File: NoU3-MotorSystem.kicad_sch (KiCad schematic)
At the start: 26 parts, among them J15 Barrel_Jack, J16 VIN, J18 GND, Q2 AONR21357, U15 SY8113BADC, U16 SY8113BADC, U8 5.8 ZSPT

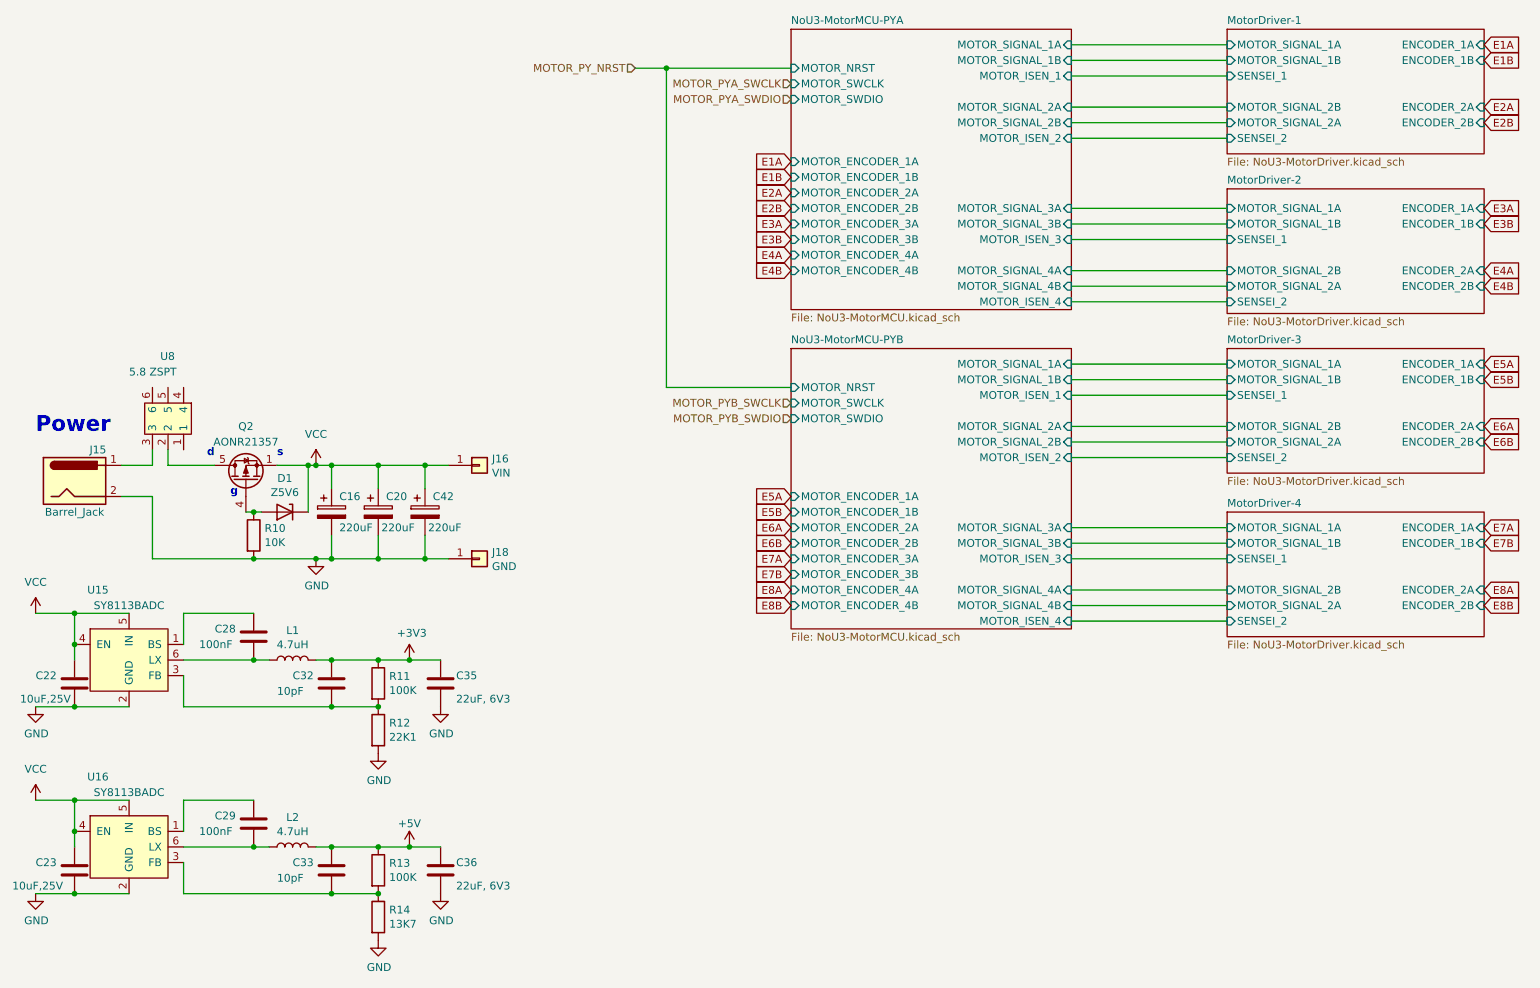
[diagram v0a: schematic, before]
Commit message: motor driver footprints
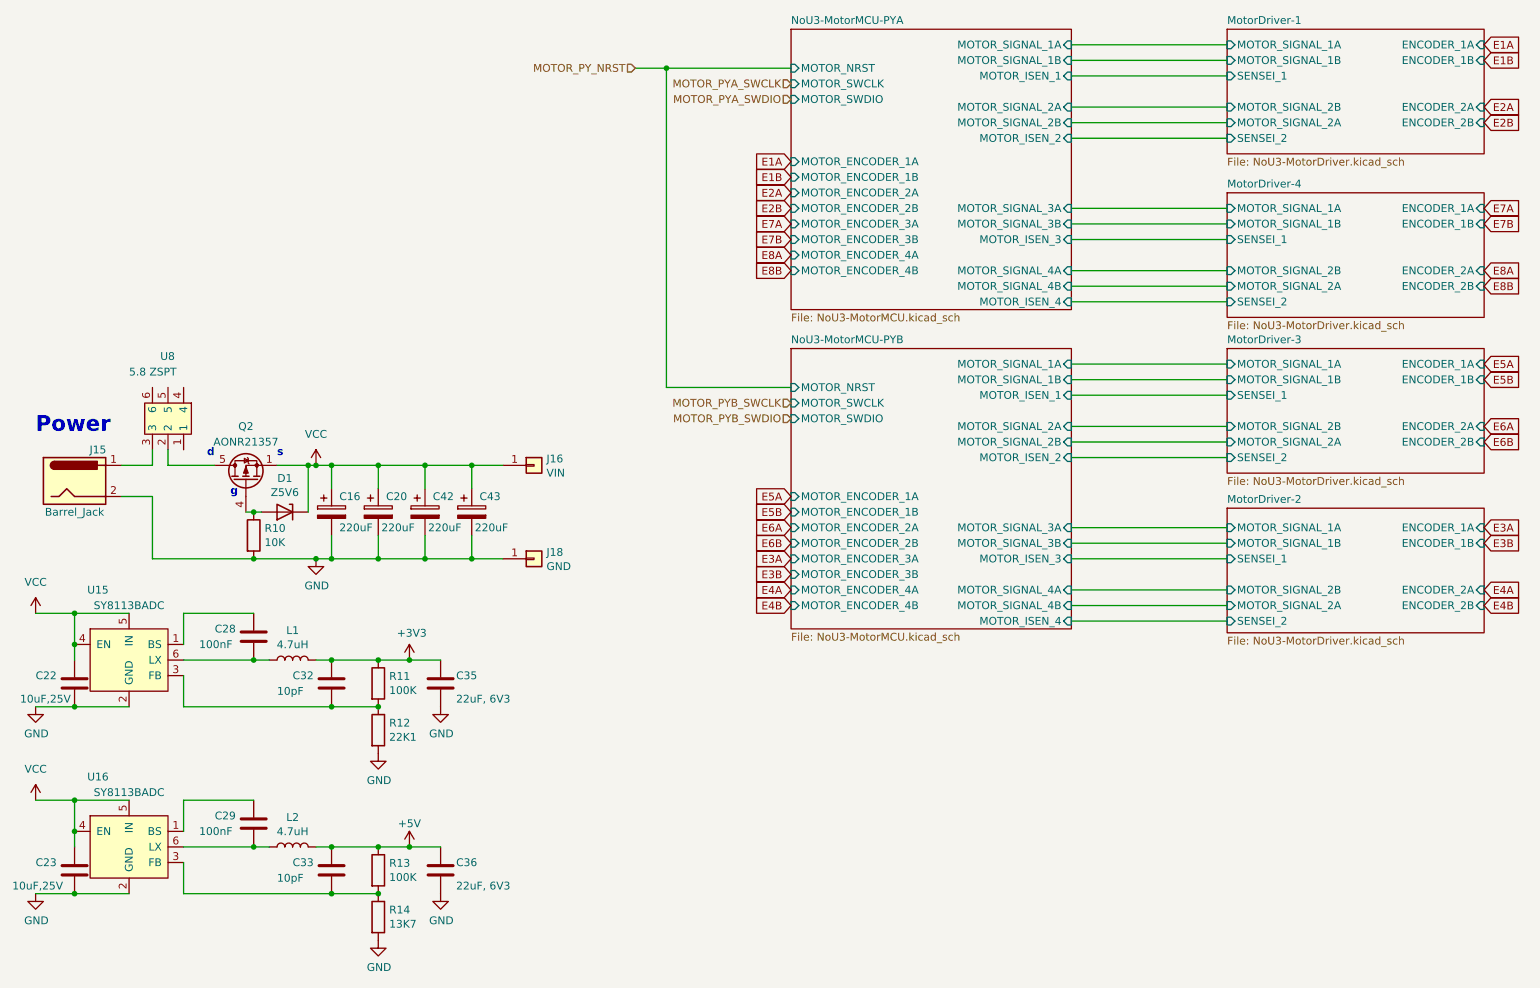
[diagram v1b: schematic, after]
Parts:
- added C43: 220uF, AlfredoFootprints:CP_Elec_6.3x7.7_slim, symbol Device:C_Polarized
- C16, C20, C42: footprint Capacitor_SMD:CP_Elec_6.3x7.7 -> AlfredoFootprints:CP_Elec_6.3x7.7_slim
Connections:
- net GND: now also C43.2
- net VCC: now also C43.1
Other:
- moved on the sheet: J16, J18
